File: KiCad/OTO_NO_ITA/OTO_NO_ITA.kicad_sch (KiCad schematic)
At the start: 0 parts

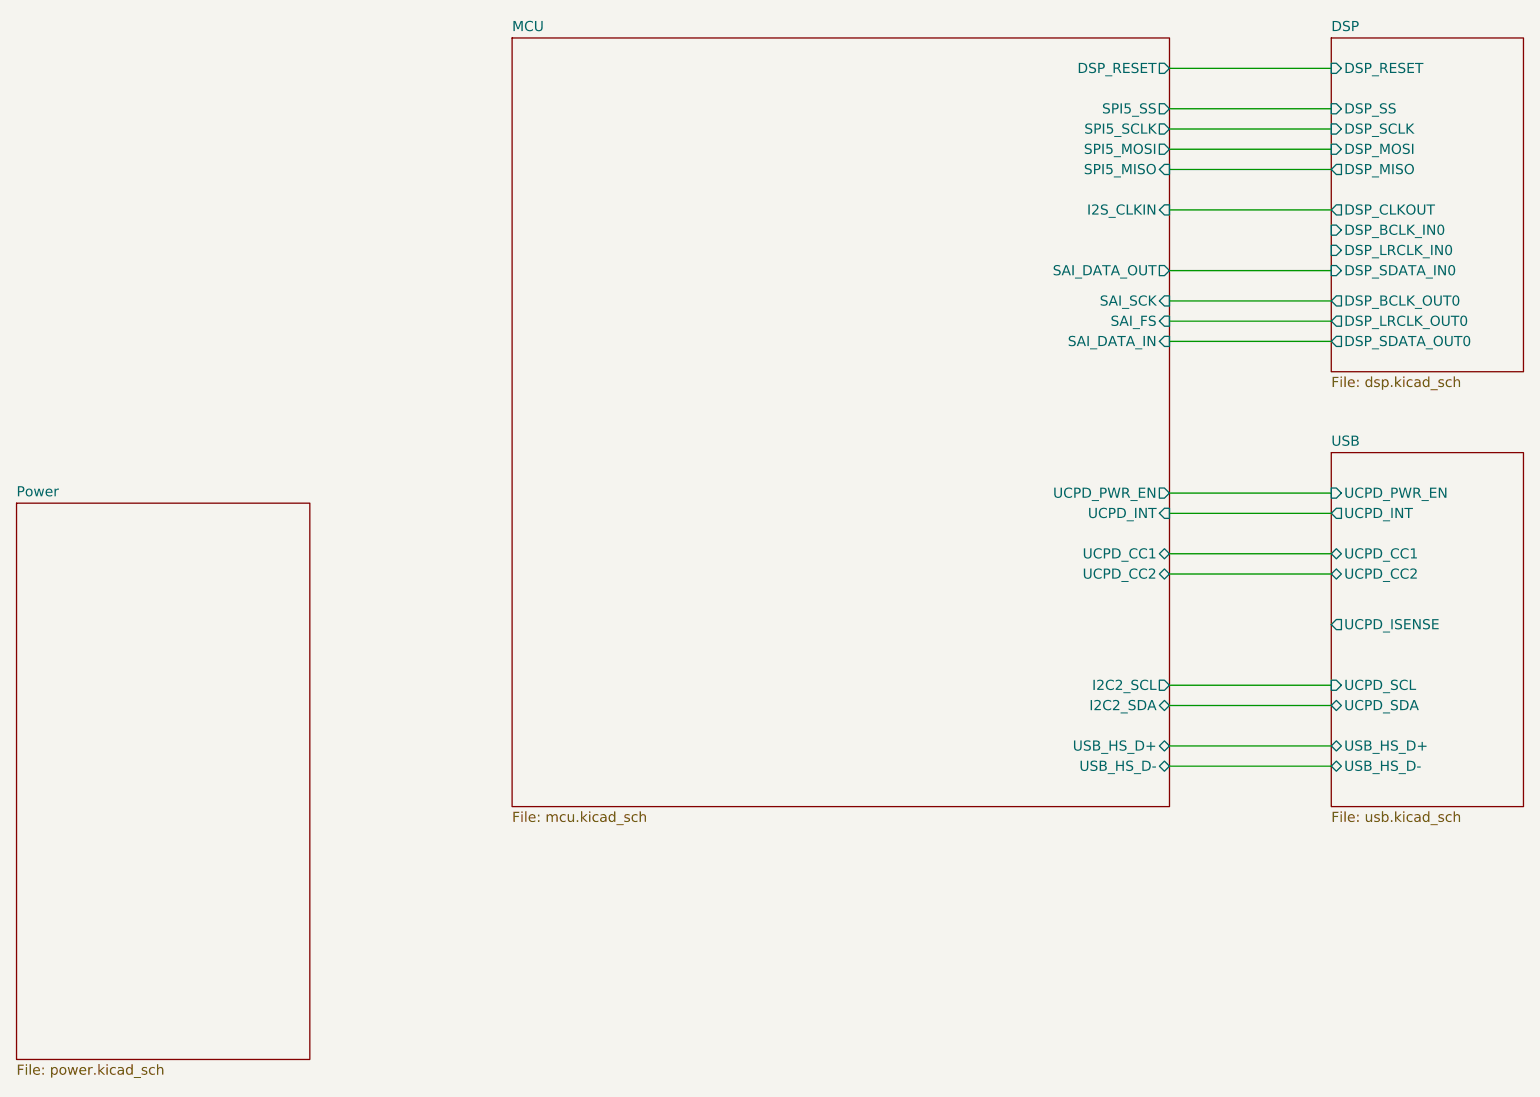
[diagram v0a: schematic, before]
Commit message: Updated schematics.
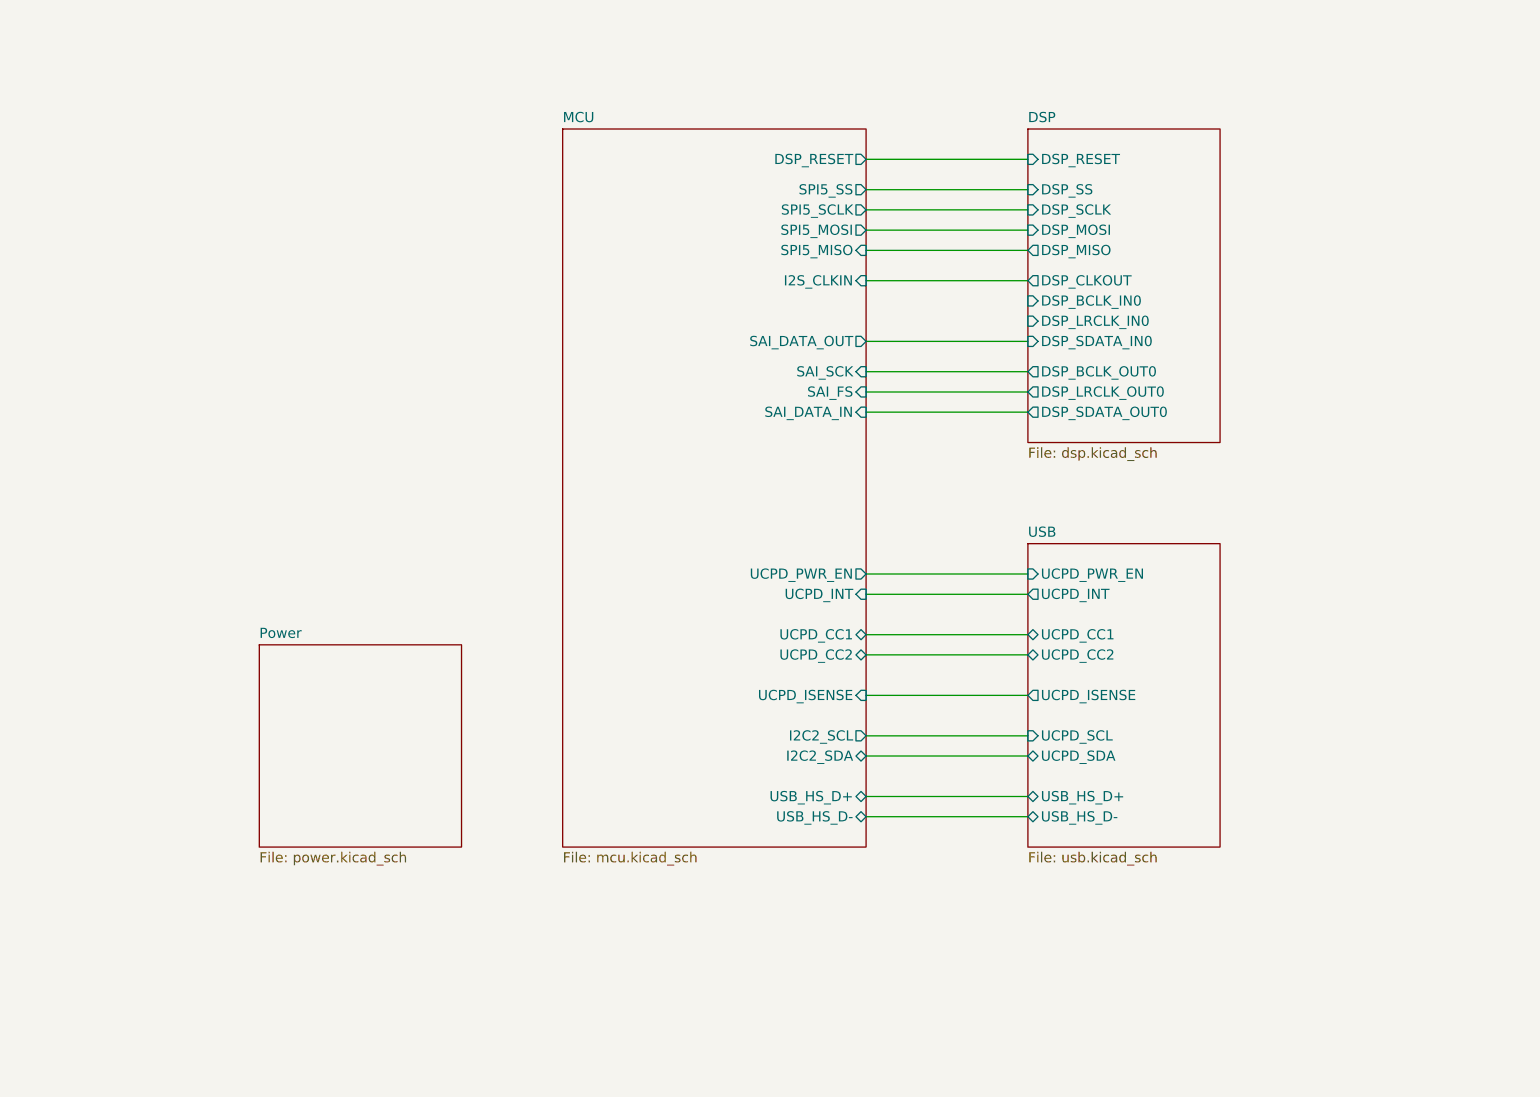
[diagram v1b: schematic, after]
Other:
- sheet MCU ports: added UCPD_ISENSE; removed none
